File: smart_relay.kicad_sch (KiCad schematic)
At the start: 8 parts, among them J2 Screw_Terminal_01x04, U1 BP8005

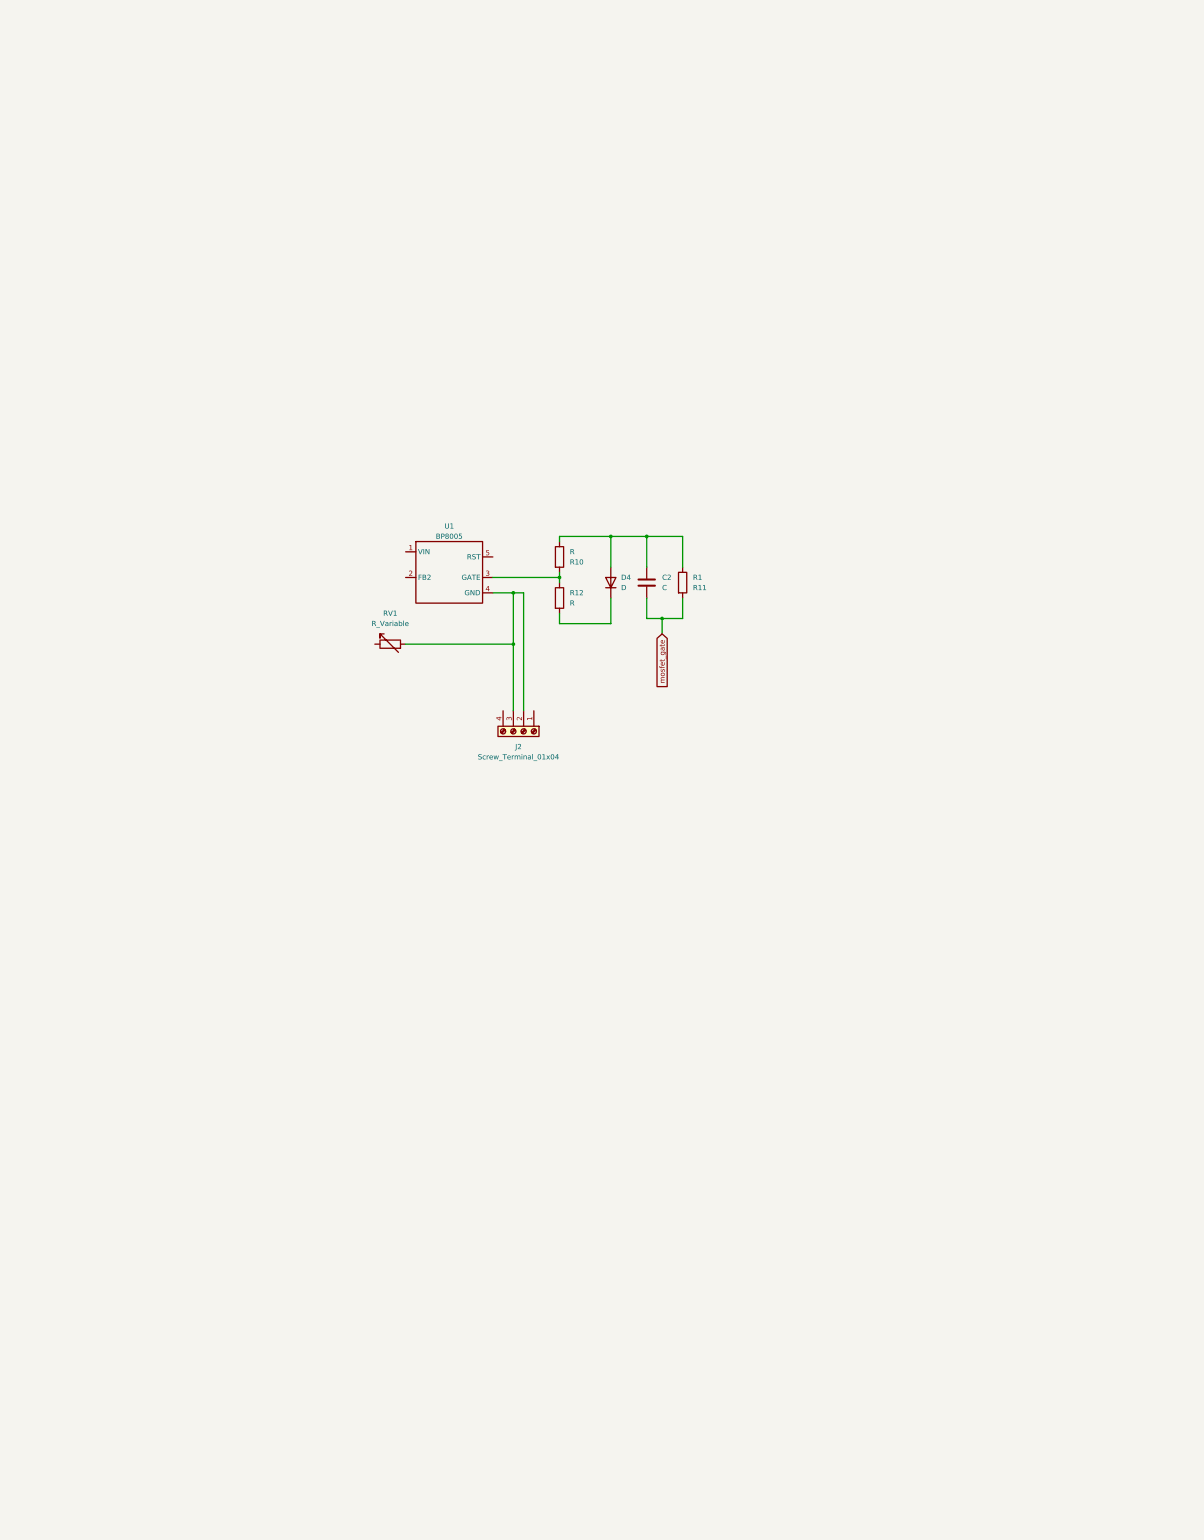
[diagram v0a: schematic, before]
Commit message: Auto commit: 2025-03-07_01-56
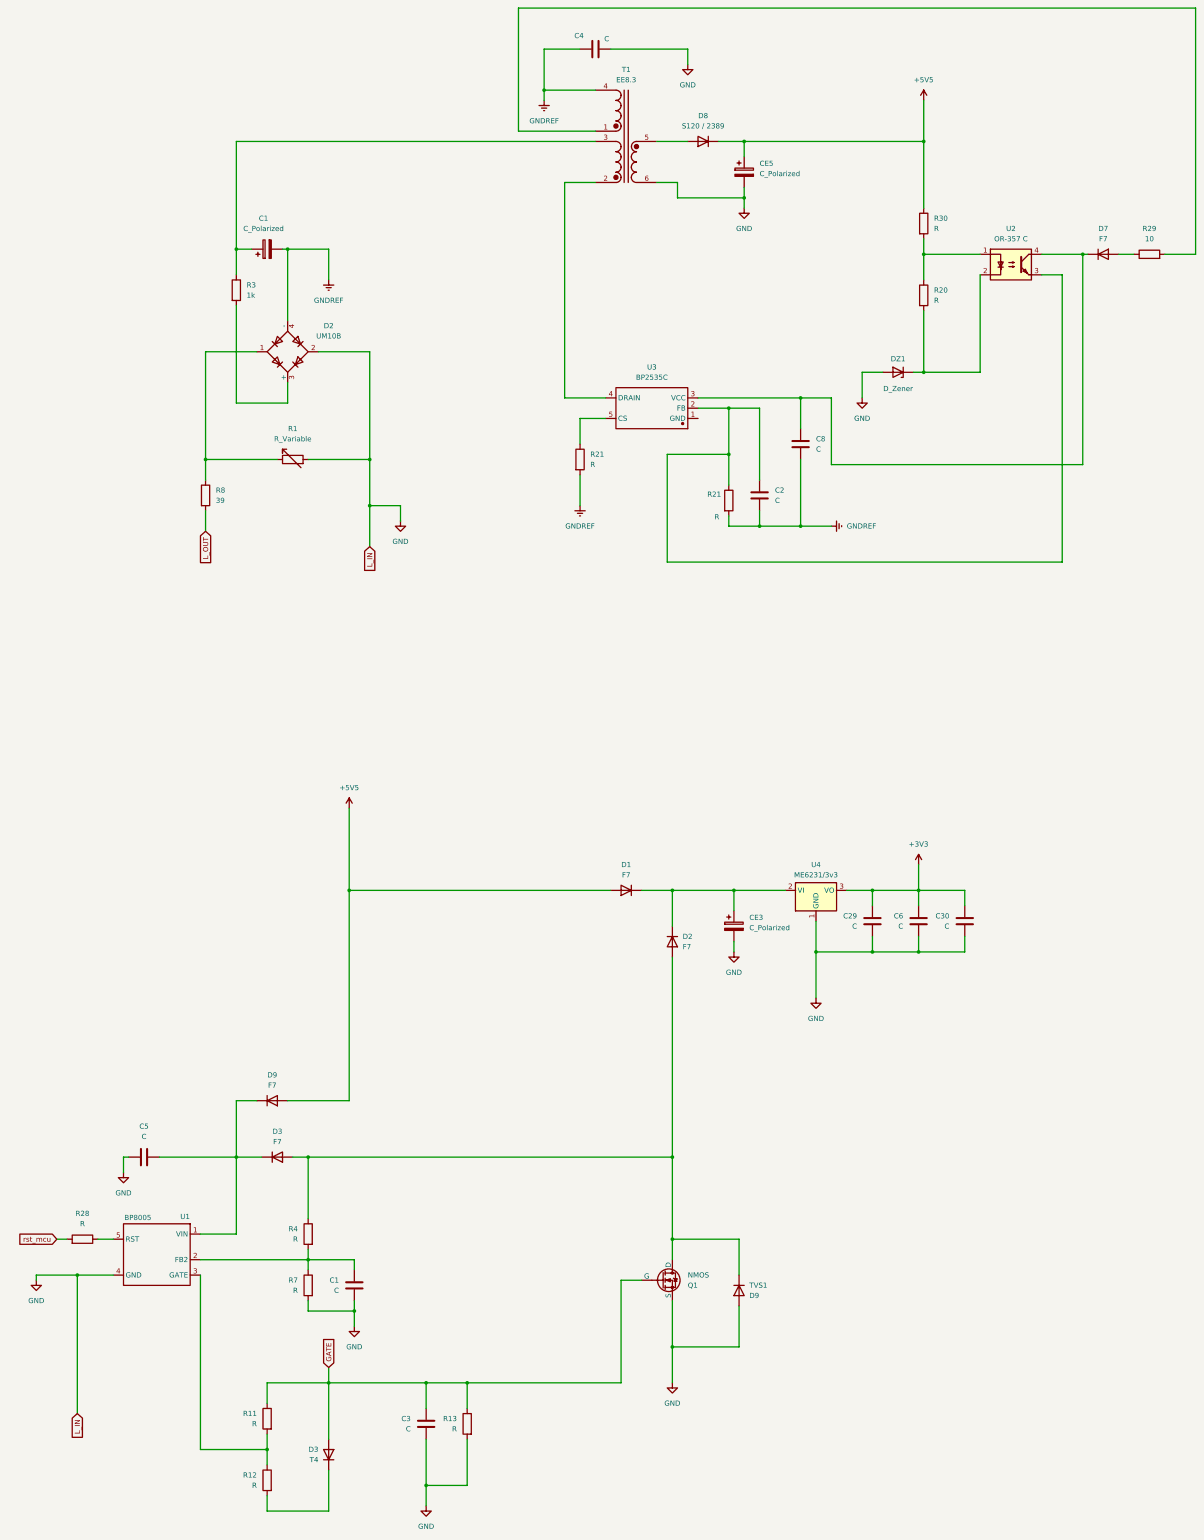
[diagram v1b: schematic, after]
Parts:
- removed D4: D, symbol Device:D
- removed J2: Screw_Terminal_01x04, TerminalBlock:TerminalBlock_MaiXu_MX126-5.0-04P_1x04_P5.00mm, symbol Connector:Screw_Terminal_01x04
- removed R: R10, symbol Device:R
- removed R1: R11, symbol Device:R
- removed RV1: R_Variable, 3225-471H:Untitled, symbol Device:R_Variable
- added C1, C29, C3, C30, C4, C5, C6, C8: C, symbol Device:C
- added C1, CE3, CE5: C_Polarized, symbol Device:C_Polarized
- added D1, D2, D3, D7, D9: F7, symbol Device:D
- added D2: UM10B, Package_TO_SOT_SMD:TO-269AA, symbol Diode_Bridge:RMB4S
- added D3: T4, symbol Device:D
- added D8: S120 / 2389, symbol Device:D
- added D9: TVS1, symbol Device:D
- added DZ1: D_Zener, symbol Device:D_Zener
- added Q1: NMOS, symbol Simulation_SPICE:NMOS
- added R1: R_Variable, symbol Device:R_Variable
- added R11, R13, R20, R21 (x2), R28, R30, R4, R7: R, symbol Device:R
- added R29: 10, symbol Device:R
- added R3: 1k, symbol Device:R
- added R8: 39, symbol Device:R
- added T1: EE8.3, symbol transformer_integrated_inductor:EE8.3
- added U2: OR-357 C, Package_DIP:DIP-4_W7.62mm, symbol Isolator:SFH617A-1
- added U3: BP2535C, symbol BP8005:BP2535C
- added U4: ME6231/3v3, Package_TO_SOT_SMD:SOT-223-3_TabPin2, symbol Regulator_Linear:AMS1117-3.3
- U1: footprint BP8005:SOT33-5B_L3.9-W2.6-P0.90-LS4.0-BL -> (none)
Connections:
- net at U1.1 (VIN): now also C5.2, D3.1 (K), D9.1 (K)
- net at U1.2 (FB2): now also C1.2, R4.2, R7.1
- net at R12.1, U1.3 (GATE): now also R11.2
- net GND: now reaches U1.4 (GND)
- net GND: now also C1.1, C29.1, C3.1, C30.1, C4.2, C5.1, C6.1, CE3.2, CE5.2, D2.2, D9.2 (A), DZ1.2 (A), Q1.3 (S), R1.2, R13.2, R7.2, T1.6 (1), U4.1 (GND)
- net at U1.5 (RST): now also R28.1
- net GNDREF: now reaches C2.1
- net GNDREF: now also C1.2, C4.1, C8.1, D2.4 (-), R21.2, R21.2, T1.4
- net at R12.2: now also D3.1 (K)
- net mosfet_gate: no longer names the net of C2.2
- net mosfet_gate: now also R21.1, U2.3, U3.2 (FB)
- new net: D2.1, R1.1, R8.1
- new net: D2.2 (A), D3.2 (A), D9.1 (K), Q1.1 (D), R4.1
- new net: DZ1.1 (K), R20.2, U2.2
- new net: CE3.1, D1.1 (K), D2.1 (K), U4.2 (VI)
- new net: C1.1, R3.1, T1.3 (6)
- new net: D2.3 (+), R3.2
- new net: D8.2 (A), T1.5 (2)
- new net: C8.2, D7.1 (K), U2.4, U3.3 (VCC)
- new net: D7.2 (A), R29.1
- new net: R20.1, R30.2, U2.1
- new net: R21.1, U3.5 (CS)
- new net: T1.2 (5), U3.4 (DRAIN)
- new net: R29.2, T1.1 (3)
- new net +3V3: C29.2, C30.2, C6.2, U4.3 (VO)
- new net +5V5: CE5.1, D1.2 (A), D8.1 (K), D9.2 (A), R30.1
- new net GATE: C3.2, D3.2 (A), Q1.2 (G), R11.1, R13.1
- new net L_OUT: R8.2
- new net rst_mcu: R28.2
